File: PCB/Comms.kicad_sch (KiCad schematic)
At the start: 23 parts, among them J2 USB_In, J3 Split_comm_link, J4 Trackpad, J5 OLED, J6 OLED_PH, U4 SRV05-4, U5 SRV05-4, U6 PMW3360DM-T2QU

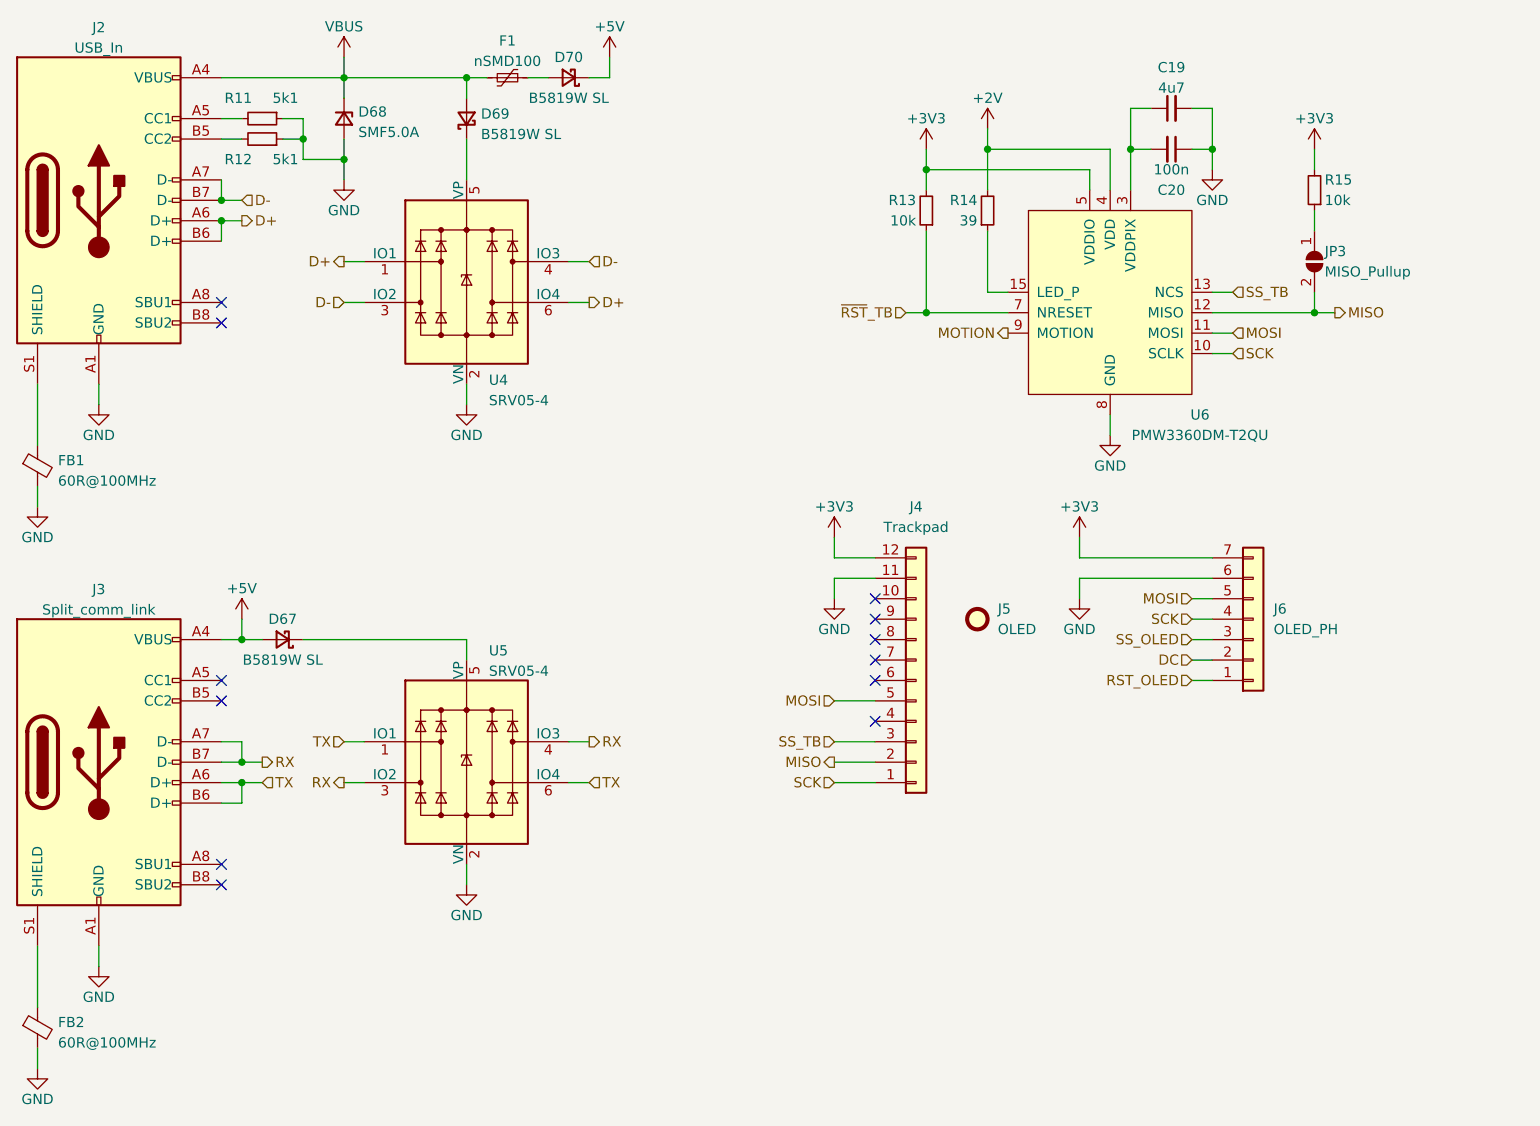
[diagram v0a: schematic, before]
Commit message: More routing
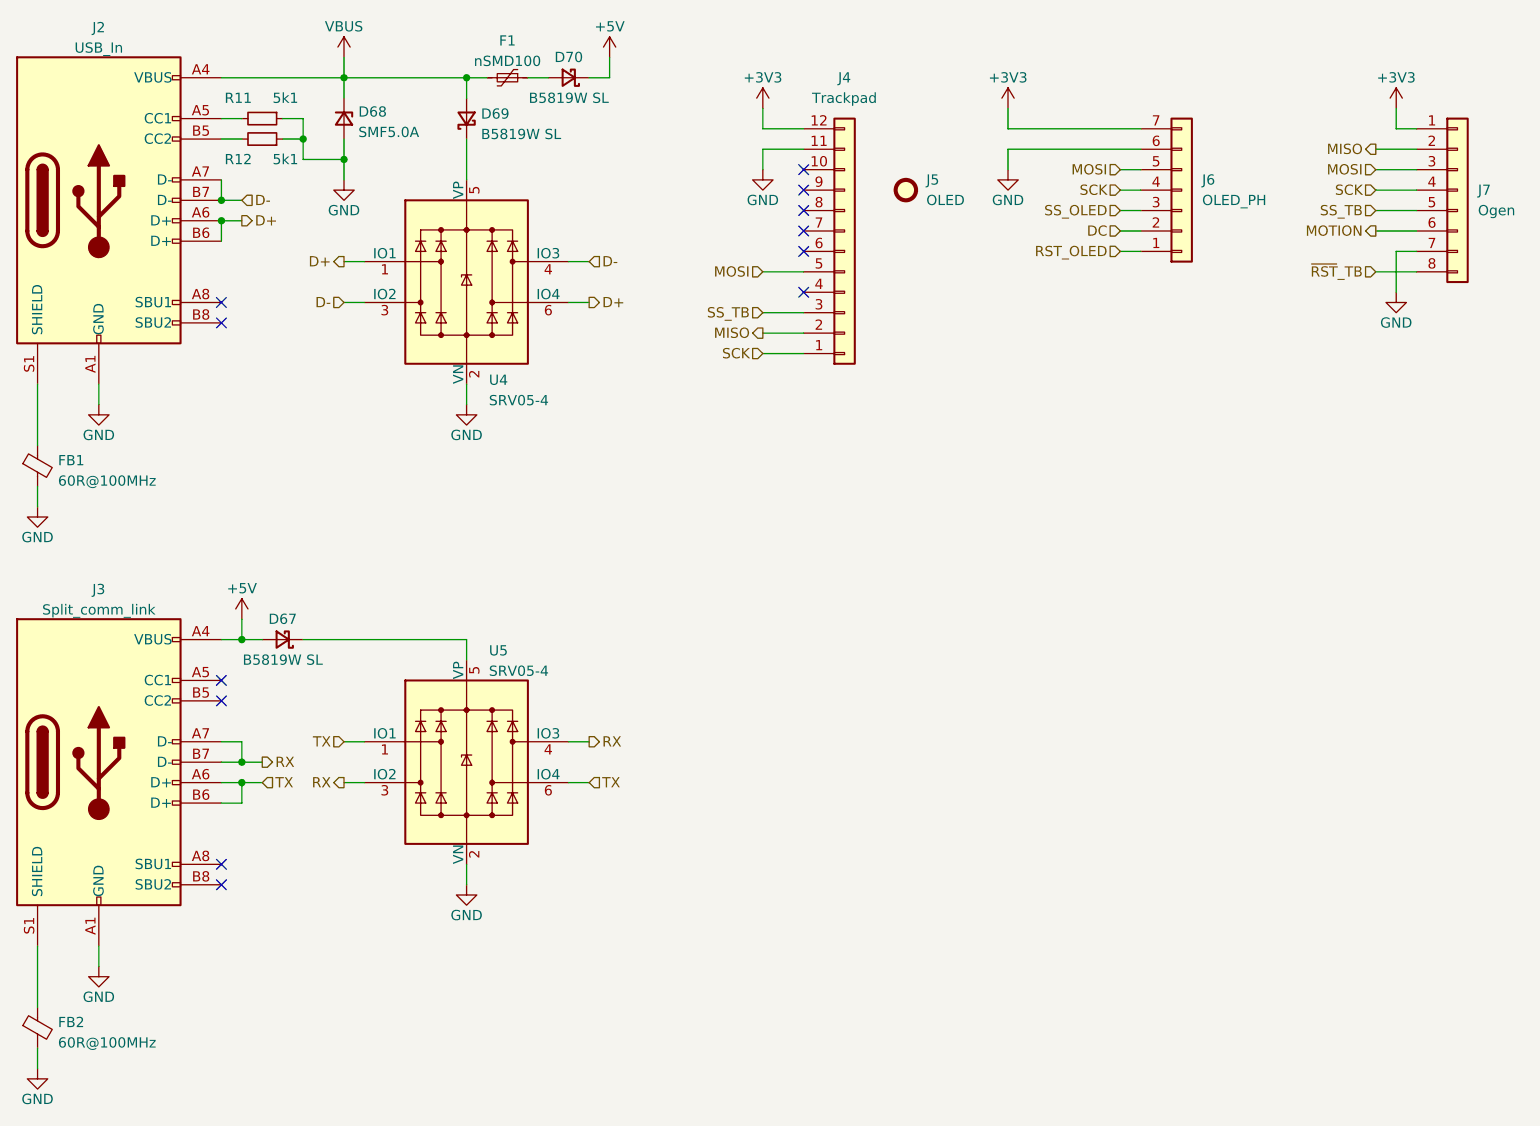
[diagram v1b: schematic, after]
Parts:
- removed C19: 4u7, Capacitor_SMD:C_0603_1608Metric, symbol Device:C_Small
- removed C20: 100n, Capacitor_SMD:C_0402_1005Metric, symbol Device:C_Small
- removed JP3: MISO_Pullup, Jumper:SolderJumper-2_P1.3mm_Open_Pad1.0x1.5mm, symbol Jumper:SolderJumper_2_Open
- removed R13, R15: 10k, Resistor_SMD:R_0402_1005Metric, symbol Device:R_Small
- removed R14: 39, Resistor_SMD:R_0402_1005Metric, symbol Device:R_Small
- removed U6: PMW3360DM-T2QU, Cantaloupe:IC_PMW3360DM-T2QU, symbol Ogen:PMW3360DM-T2QU
- added J7: Ogen, Cantaloupe:Ogen-Flippable, symbol Connector_Generic:Conn_01x08
- J6: footprint Cantaloupe:JST_PH_S7B-PH-K_1x07_P2.00mm_Horizontal-Dual -> Cantaloupe:JST_PH_S7B-PH-K_1x07_P2.00mm_Horizontal-Flippable
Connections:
- net +3V3: now also J7.1 (Pin_1)
- net GND: now also J7.7 (Pin_7)
- net MISO: now also J7.2 (Pin_2)
- net MOSI: now also J7.3 (Pin_3)
- net MOTION: now also J7.6 (Pin_6)
- net SCK: now also J7.4 (Pin_4)
- net SS_TB: now also J7.5 (Pin_5)
- net ~{RST}_TB: now also J7.8 (Pin_8)
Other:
- moved on the sheet: J4, J5, J6
